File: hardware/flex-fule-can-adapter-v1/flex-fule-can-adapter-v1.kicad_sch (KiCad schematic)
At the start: 38 parts, among them J1 Ethanol Sensor, J2 CAR, SW1 RESET, SW2 BOOT, U1 ESP32-C3-WROOM-02U-N4, U2 SN65HVD230QDR, U3 TPS259472ARPWR, U4 TPS62901RPJR

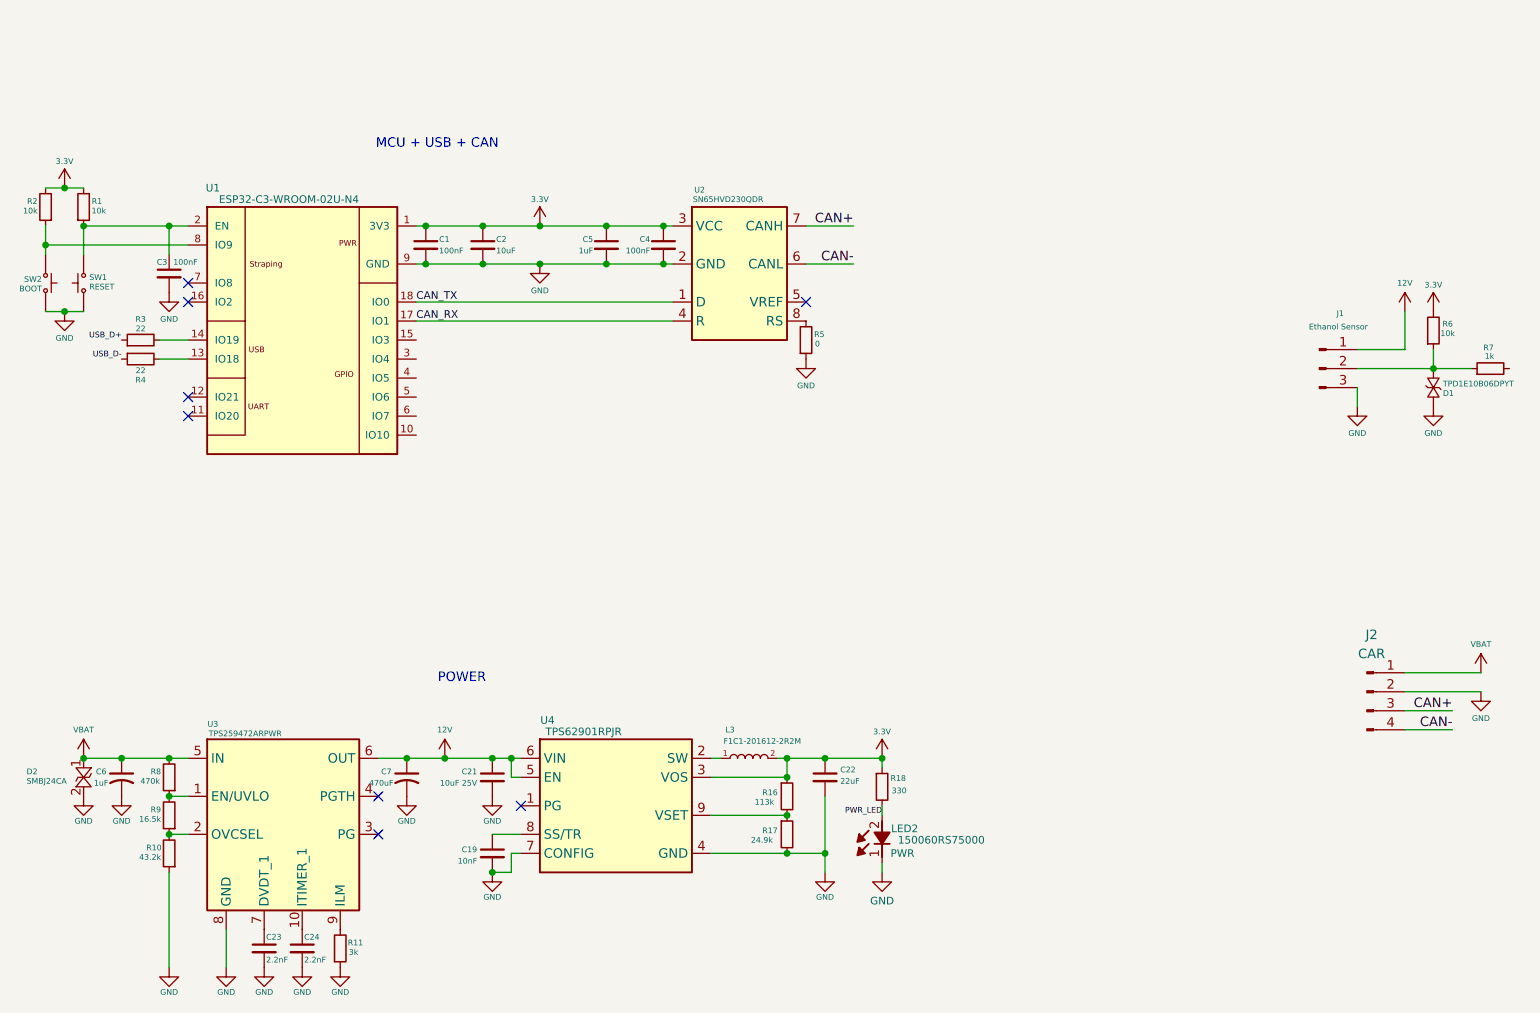
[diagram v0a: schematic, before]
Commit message: Sch done
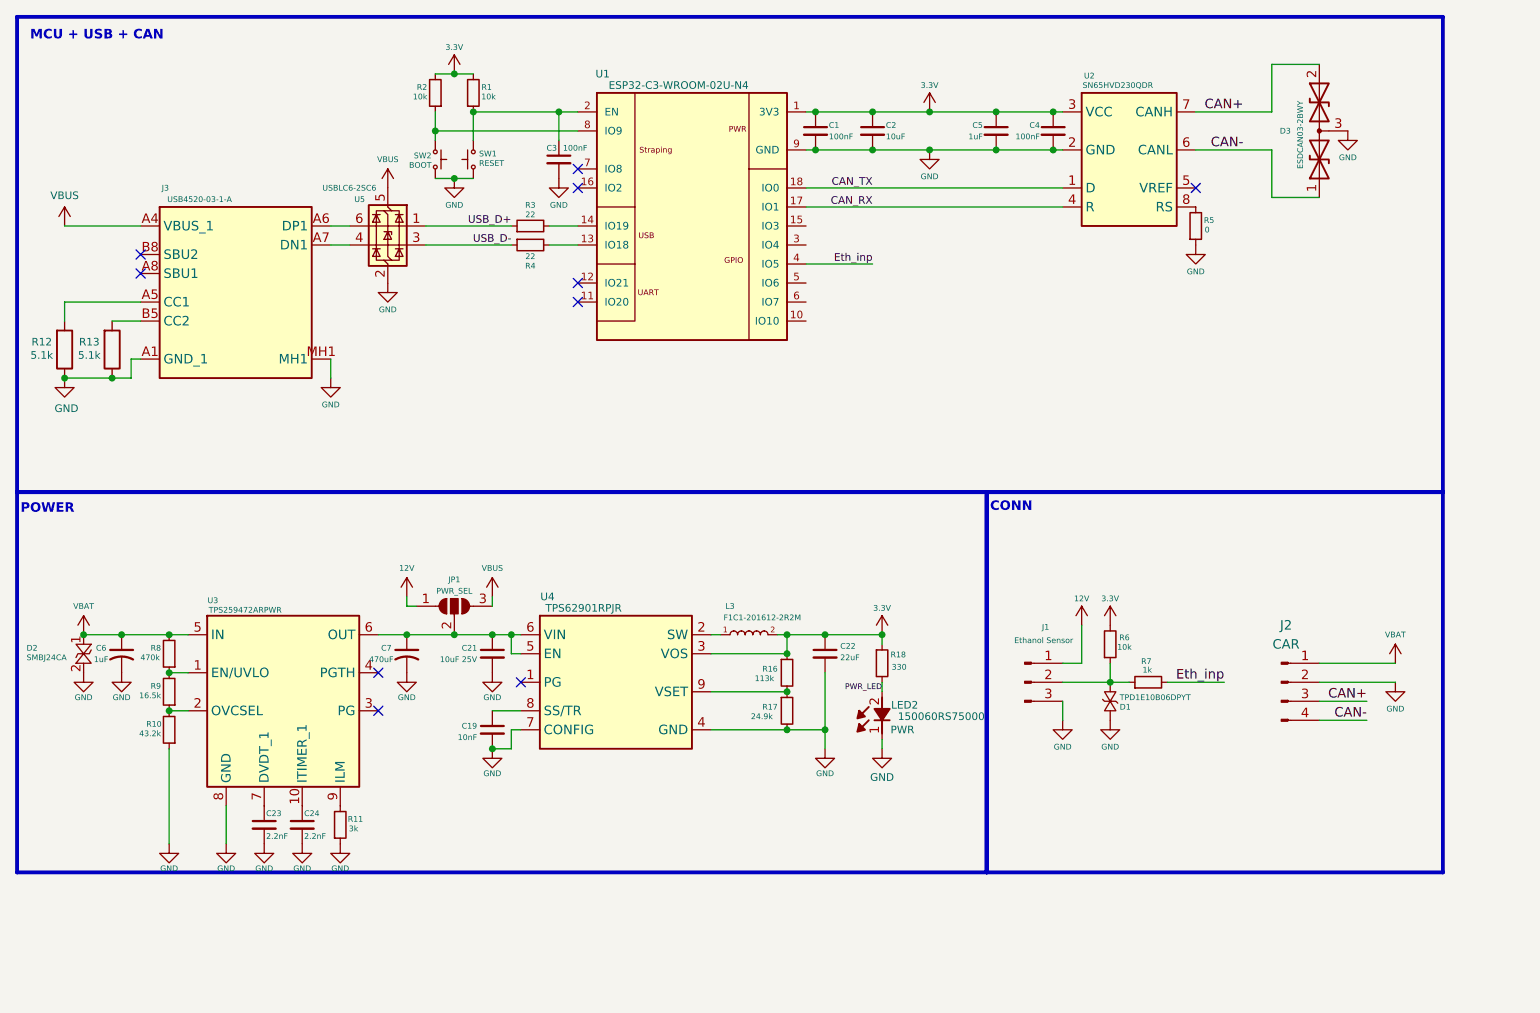
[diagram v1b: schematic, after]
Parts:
- added D3: ESDCAN03-2BWY, SDM_MiscFootprint:SOT65P210X110-3N, symbol SDM_DIODES:ESDCAN03-2BWY
- added J3: USB4520-03-1-A, ModLib:USB4520031A, symbol SchLib:USB4520-03-1-A
- added JP1: PWR_SEL, Jumper:SolderJumper-3_P1.3mm_Open_RoundedPad1.0x1.5mm_NumberLabels, symbol Jumper:SolderJumper_3_Open
- added R12, R13: 5.1k, Resistor_SMD:R_0603_1608Metric, symbol Device:R
- added U5: USBLC6-2SC6, Package_TO_SOT_SMD:SOT-23-6, symbol Power_Protection:USBLC6-2SC6
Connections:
- net 12V: now also JP1.1 (A); no longer C21.1, C7.1, U3.6 (OUT), U4.5 (EN), U4.6 (VIN)
- net CAN+: now also D3.2
- net CAN-: now also D3.1
- net GND: now also D3.3, J3.A1 (GND_1), J3.A12 (GND_2), J3.MH1, J3.MH2, J3.MH3, J3.MH4, R12.1, R13.1, U5.2 (GND)
- net USB_D+: now also U5.1 (I/O1)
- net USB_D-: now also U5.3 (I/O2)
- net Eth_inp: now reaches R7.2
- net Eth_inp: now also U1.4 (IO5)
- new net: J3.A7 (DN1), J3.B7 (DN2), U5.4 (I/O2)
- new net: J3.A6 (DP1), J3.B6 (DP2), U5.6 (I/O1)
- new net: C21.1, C7.1, JP1.2 (C), U3.6 (OUT), U4.5 (EN), U4.6 (VIN)
- new net: J3.A5 (CC1), R12.2
- new net: J3.B5 (CC2), R13.2
- new net VBUS: J3.A4 (VBUS_1), J3.A9 (VBUS_2), JP1.3 (B), U5.5 (VBUS)
- no-connect marks 8 -> 10
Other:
- note added: "CONN"
- moved on the sheet: C1, C19, C2, C21, C22, C23, C24, C3, C4, C5, C6, C7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
